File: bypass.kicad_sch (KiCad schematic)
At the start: 8 parts

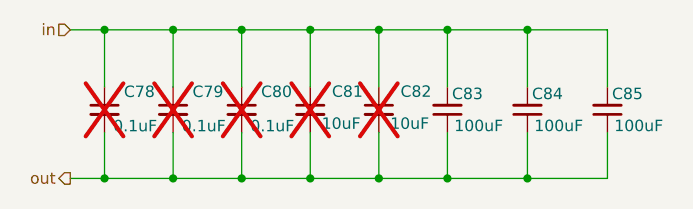
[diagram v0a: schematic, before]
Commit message: run through ERC
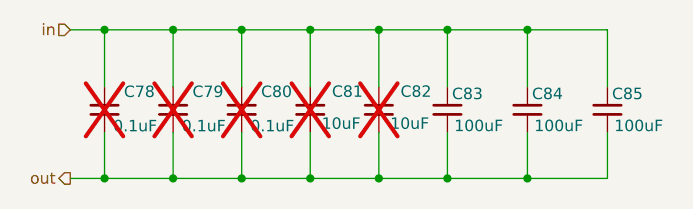
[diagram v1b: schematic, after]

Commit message: switched 100uF ASIC domain bypass caps to cheaper 1206
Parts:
- C83, C84, C85: footprint Capacitor_SMD:C_0805_2012Metric -> Capacitor_SMD:C_1206_3216Metric; DK 490-GRM21BR60G107ME11KCT-ND -> 1276-1782-1-ND; LCSC C7282454 -> C15008; PARTNO GRM21BR60G107ME11K -> CL31A107MQHNNNE
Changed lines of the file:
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@@
 			)
 		)
-		(property "Footprint" "Capacitor_SMD:C_0805_2012Metric"
+		(property "Footprint" "Capacitor_SMD:C_1206_3216Metric"
 			(at 175.26 82.55 0)
 			(hide yes)
@@
 			)
 		)
-		(property "PARTNO" "GRM21BR60G107ME11K"
+		(property "PARTNO" "CL31A107MQHNNNE"
 			(at 175.26 82.55 0)
 			(hide yes)
@@
 			)
 		)
-		(property "DK" "490-GRM21BR60G107ME11KCT-ND"
+		(property "DK" "1276-1782-1-ND"
 			(at 175.26 82.55 0)
 			(hide yes)
@@
 			)
 		)
-		(property "LCSC" "C7282454"
+		(property "LCSC" "C15008"
 			(at 175.26 82.55 0)
 			(hide yes)
@@
 			)
 		)
-		(property "Footprint" "Capacitor_SMD:C_0805_2012Metric"
+		(property "Footprint" "Capacitor_SMD:C_1206_3216Metric"
 			(at 166.37 82.55 0)
 			(hide yes)
@@
 			)
 		)
-		(property "PARTNO" "GRM21BR60G107ME11K"
+		(property "PARTNO" "CL31A107MQHNNNE"
 			(at 166.37 82.55 0)
 			(hide yes)
@@
 			)
 		)
-		(property "DK" "490-GRM21BR60G107ME11KCT-ND"
+		(property "DK" "1276-1782-1-ND"
 			(at 166.37 82.55 0)
 			(hide yes)
@@
 			)
 		)
-		(property "LCSC" "C7282454"
+		(property "LCSC" "C15008"
 			(at 166.37 82.55 0)
 			(hide yes)
@@
 			)
 		)
-		(property "Footprint" "Capacitor_SMD:C_0805_2012Metric"
+		(property "Footprint" "Capacitor_SMD:C_1206_3216Metric"
 			(at 157.48 82.55 0)
 			(hide yes)
@@
 			)
 		)
-		(property "PARTNO" "GRM21BR60G107ME11K"
+		(property "PARTNO" "CL31A107MQHNNNE"
 			(at 157.48 82.55 0)
 			(hide yes)
@@
 			)
 		)
-		(property "DK" "490-GRM21BR60G107ME11KCT-ND"
+		(property "DK" "1276-1782-1-ND"
 			(at 157.48 82.55 0)
 			(hide yes)
@@
 			)
 		)
-		(property "LCSC" "C7282454"
+		(property "LCSC" "C15008"
 			(at 157.48 82.55 0)
 			(hide yes)
